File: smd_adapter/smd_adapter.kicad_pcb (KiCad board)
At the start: 2 copper layers, 63.9 x 74.2 mm, 260 parts, among them J1 Conn_01x01_Pin, J10 Conn_01x01_Pin, J11 Conn_01x01_Pin, J12 Conn_01x01_Pin, J13 Conn_01x01_Pin, J14 Conn_01x01_Pin, J15 Conn_01x01_Pin, J16 Conn_01x01_Pin, J17 Conn_01x01_Pin, J18 Conn_01x01_Pin, J19 Conn_01x01_Pin, J2 Conn_01x01_Pin, J20 Conn_01x01_Pin, J21 Conn_01x01_Pin, J22 Conn_01x01_Pin, J23 Conn_01x01_Pin, J24 Conn_01x01_Pin, J25 Conn_01x01_Pin, J26 Conn_01x01_Pin, J27 Conn_01x01_Pin, J28 Conn_01x01_Pin, J29 Conn_01x01_Pin, J3 Conn_01x01_Pin, J30 Conn_01x01_Pin, J31 Conn_01x01_Pin, J32 Conn_01x01_Pin, J33 Conn_01x01_Pin, J34 Conn_01x01_Pin, J35 Conn_01x01_Pin, J36 Conn_01x01_Pin, J37 Conn_01x01_Pin, J4 Conn_01x01_Pin, J5 Conn_01x01_Pin, J6 Conn_01x01_Pin, J7 Conn_01x01_Pin, J8 Conn_01x01_Pin, J9 Conn_01x01_Pin, U1 SOIC8, U2 SOT_32-5, U3 SOT_32-6, U4 MSOP8, U5 TSSOP-10

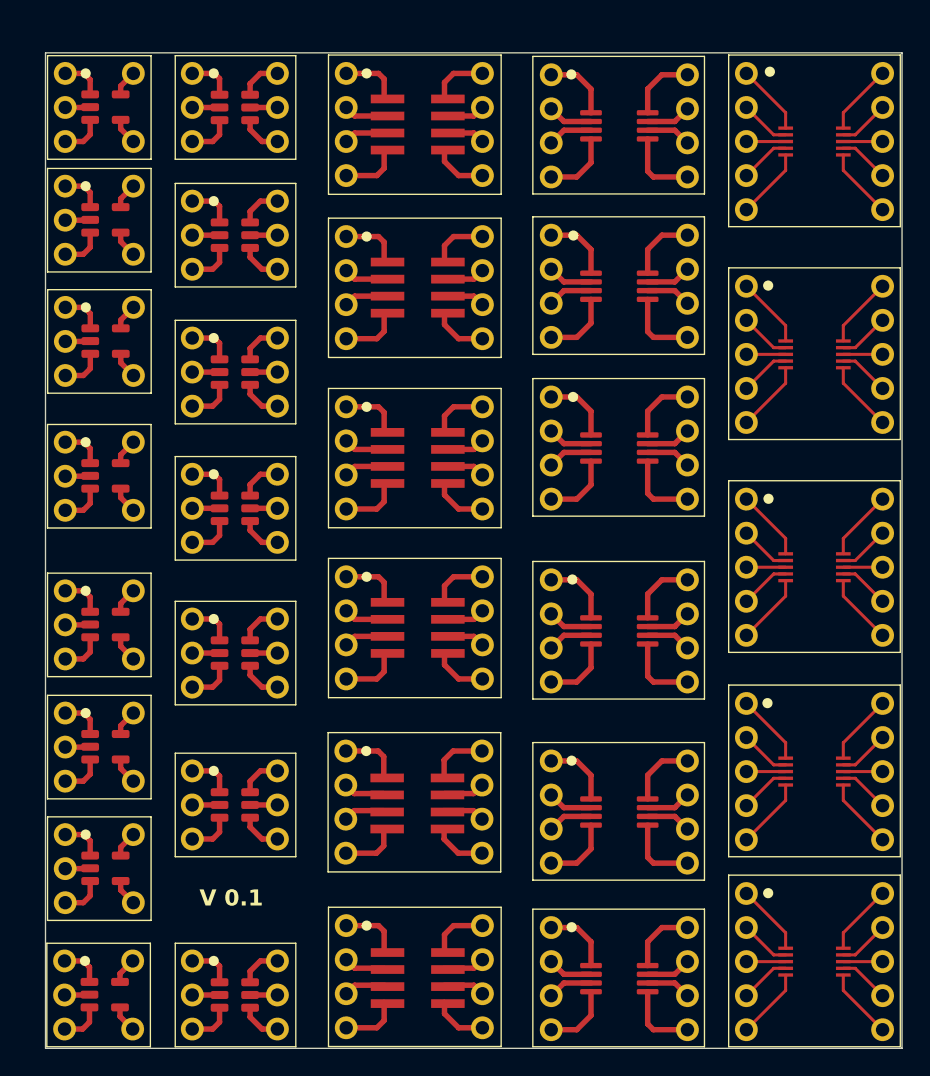
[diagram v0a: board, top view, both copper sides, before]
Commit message: Generated production files.
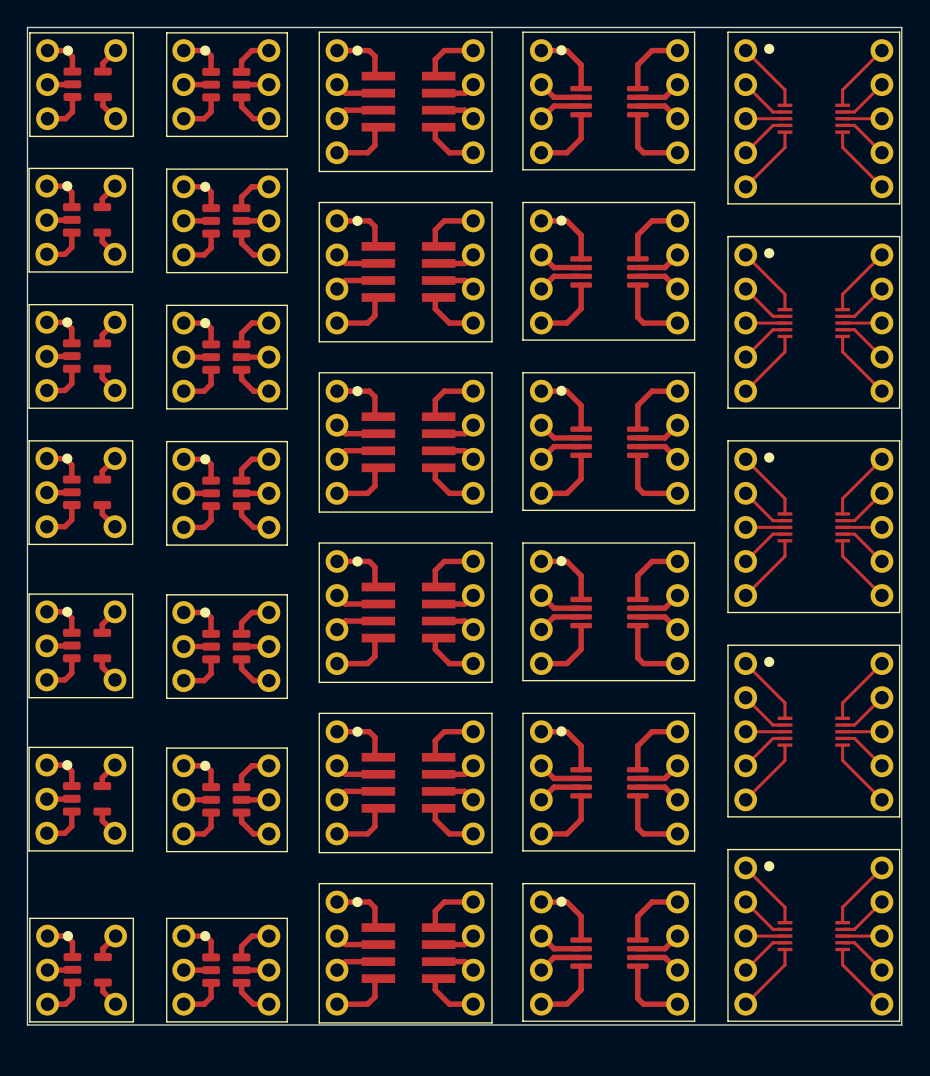
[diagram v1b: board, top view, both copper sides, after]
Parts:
- removed the J1 at (87.7, 107.8)
- removed the J1 at (87.6, 126.3)
- removed the J1 at (87.7, 87.6)
- removed the J1 at (87.7, 68.5)
- removed the J1 at (87.7, 98.7)
- removed the J1 at (87.7, 116.9)
- removed the J1 at (87.7, 77.6)
- removed the J10 at (113.7, 105.6)
- removed the J10 at (113.7, 118.6)
- removed the J10 at (113.7, 79.9)
- removed the J10 at (113.7, 92.6)
- removed the J10 at (113.7, 67.2)
- removed the J11 at (113.7, 82.4)
- removed the J11 at (113.7, 95.1)
- removed the J11 at (113.7, 69.7)
- removed the J11 at (113.7, 121.1)
- removed the J11 at (113.7, 108.1)
- removed the J12 at (113.7, 110.7)
- removed the J12 at (113.7, 85.0)
- removed the J12 at (113.7, 97.7)
- removed the J12 at (113.7, 72.3)
- removed the J12 at (113.7, 123.7)
- removed the J13 at (113.7, 113.2)
- removed the J13 at (113.7, 87.5)
- removed the J13 at (113.7, 74.8)
- removed the J13 at (113.7, 100.2)
- removed the J13 at (113.7, 126.2)
- removed the J14 at (92.1, 121.2)
- removed the J14 at (92.1, 64.6)
- removed the J14 at (92.1, 95.7)
- removed the J14 at (92.1, 107.1)
- removed the J14 at (92.1, 74.8)
- removed the J14 at (92.1, 84.9)
- removed the J15 at (92.1, 98.3)
- removed the J15 at (92.1, 109.6)
- removed the J15 at (92.1, 123.8)
- removed the J15 at (92.1, 77.3)
- removed the J15 at (92.1, 87.5)
- removed the J15 at (92.1, 67.1)
- removed the J16 at (92.1, 112.1)
- removed the J16 at (92.1, 126.3)
- removed the J16 at (92.1, 69.6)
- removed the J16 at (92.1, 90.0)
- removed the J16 at (92.1, 79.9)
- removed the J16 at (92.1, 100.8)
- removed the J17 at (98.4, 74.8)
- removed the J17 at (98.4, 121.2)
- removed the J17 at (98.4, 95.7)
- removed the J17 at (98.4, 84.9)
- removed the J17 at (98.4, 64.6)
- removed the J17 at (98.4, 107.1)
- removed the J18 at (98.4, 109.6)
- removed the J18 at (98.4, 77.3)
- removed the J18 at (98.4, 98.3)
- removed the J18 at (98.4, 123.8)
- removed the J18 at (98.4, 87.5)
- removed the J18 at (98.4, 67.1)
- removed the J19 at (98.4, 100.8)
- removed the J19 at (98.4, 126.3)
- removed the J19 at (98.4, 79.9)
- removed the J19 at (98.4, 69.6)
- removed the J19 at (98.4, 90.0)
- removed the J19 at (98.4, 112.1)
- removed the J2 at (87.7, 72.5)
- removed the J2 at (87.7, 82.5)
- removed the J2 at (87.7, 63.4)
- removed the J2 at (87.7, 93.6)
- removed the J2 at (87.6, 121.2)
- removed the J2 at (87.7, 102.7)
- removed the J2 at (87.7, 111.8)
- removed the J20 at (118.8, 79.2)
- removed the J20 at (118.8, 67.1)
- removed the J20 at (118.8, 118.7)
- removed the J20 at (118.8, 106.3)
- removed the J20 at (118.8, 92.8)
- removed the J21 at (118.8, 81.7)
- removed the J21 at (118.8, 69.6)
- removed the J21 at (118.8, 108.9)
- removed the J21 at (118.8, 95.4)
- removed the J21 at (118.8, 121.3)
- removed the J22 at (118.8, 123.8)
- removed the J22 at (118.8, 111.4)
- removed the J22 at (118.8, 97.9)
- removed the J22 at (118.8, 84.3)
- removed the J22 at (118.8, 72.2)
- removed the J23 at (118.8, 126.4)
- removed the J23 at (118.8, 74.7)
- removed the J23 at (118.8, 86.8)
- removed the J23 at (118.8, 100.4)
- removed the J23 at (118.8, 113.9)
- removed the J24 at (129.0, 118.7)
- removed the J24 at (129.0, 67.1)
- removed the J24 at (129.0, 106.3)
- removed the J24 at (129.0, 79.2)
- removed the J24 at (129.0, 92.8)
- removed the J25 at (129.0, 81.7)
- removed the J25 at (129.0, 95.4)
- removed the J25 at (129.0, 69.6)
- removed the J25 at (129.0, 121.3)
- removed the J25 at (129.0, 108.9)
- removed the J26 at (129.0, 123.8)
- removed the J26 at (129.0, 97.9)
- removed the J26 at (129.0, 72.2)
- removed the J26 at (129.0, 111.4)
- removed the J26 at (129.0, 84.3)
- removed the J27 at (129.0, 86.8)
- removed the J27 at (129.0, 126.4)
- removed the J27 at (129.0, 74.7)
- removed the J27 at (129.0, 113.9)
- removed the J27 at (129.0, 100.4)
- removed the J28 at (133.4, 70.9)
- removed the J28 at (133.4, 86.8)
- removed the J28 at (133.4, 116.2)
- removed the J28 at (133.4, 102.0)
- removed the J29 at (133.4, 104.6)
- removed the J29 at (133.4, 118.7)
- removed the J29 at (133.4, 73.5)
- removed the J29 at (133.4, 89.3)
- removed the J3 at (82.6, 96.2)
- removed the J3 at (82.6, 114.4)
- removed the J3 at (82.6, 75.0)
- removed the J3 at (82.6, 66.0)
- removed the J3 at (82.5, 123.8)
- removed the J3 at (82.6, 105.3)
- removed the J3 at (82.6, 85.1)
- removed the J30 at (133.4, 107.1)
- removed the J30 at (133.4, 91.9)
- removed the J30 at (133.4, 121.3)
- removed the J30 at (133.4, 76.0)
- removed the J31 at (133.4, 109.7)
- removed the J31 at (133.4, 123.8)
- removed the J31 at (133.4, 94.4)
- removed the J31 at (133.4, 78.5)
- removed the J32 at (133.4, 81.1)
- removed the J32 at (133.4, 126.4)
- removed the J32 at (133.4, 112.2)
- removed the J32 at (133.4, 97.0)
- removed the J33 at (143.6, 102.0)
- removed the J33 at (143.6, 116.2)
- removed the J33 at (143.6, 70.9)
- removed the J33 at (143.6, 86.8)
- removed the J34 at (143.6, 118.7)
- removed the J34 at (143.6, 104.6)
- removed the J34 at (143.6, 89.3)
- removed the J34 at (143.6, 73.5)
- removed the J35 at (143.6, 121.3)
- removed the J35 at (143.6, 91.9)
- removed the J35 at (143.6, 107.1)
- removed the J35 at (143.6, 76.0)
- removed the J36 at (143.6, 78.5)
- removed the J36 at (143.6, 109.7)
- removed the J36 at (143.6, 123.8)
- removed the J36 at (143.6, 94.4)
- removed the J37 at (143.6, 112.2)
- removed the J37 at (143.6, 126.4)
- removed the J37 at (143.6, 97.0)
- removed the J37 at (143.6, 81.1)
- removed the J4 at (82.6, 102.7)
- removed the J4 at (82.6, 111.8)
- removed the J4 at (82.6, 63.4)
- removed the J4 at (82.5, 121.2)
- removed the J4 at (82.6, 82.5)
- removed the J4 at (82.6, 72.5)
- removed the J4 at (82.6, 93.6)
- removed the J5 at (82.6, 87.6)
- removed the J5 at (82.6, 116.9)
- removed the J5 at (82.6, 68.5)
- removed the J5 at (82.6, 77.6)
- removed the J5 at (82.6, 98.7)
- removed the J5 at (82.5, 126.3)
- removed the J5 at (82.6, 107.8)
- removed the J6 at (103.5, 105.6)
- removed the J6 at (103.6, 67.2)
- removed the J6 at (103.6, 92.6)
- removed the J6 at (103.6, 118.6)
- removed the J6 at (103.6, 79.9)
- removed the J7 at (103.6, 121.1)
- removed the J7 at (103.5, 108.1)
- removed the J7 at (103.6, 95.1)
- removed the J7 at (103.6, 69.7)
- removed the J7 at (103.6, 82.4)
- removed the J8 at (103.6, 123.7)
- removed the J8 at (103.5, 110.7)
- removed the J8 at (103.6, 85.0)
- removed the J8 at (103.6, 97.7)
- removed the J8 at (103.6, 72.3)
- removed the J9 at (103.5, 113.2)
- removed the J9 at (103.6, 74.8)
- removed the J9 at (103.6, 87.5)
- removed the J9 at (103.6, 100.2)
- removed the J9 at (103.6, 126.2)
- removed the U1 at (108.9, 71.0)
- removed the U1 at (108.9, 109.5)
- removed the U1 at (108.9, 122.5)
- removed the U1 at (108.9, 83.7)
- removed the U1 at (108.9, 96.4)
- removed the U2 at (85.6, 85.1)
- removed the U2 at (85.6, 114.3)
- removed the U2 at (85.5, 123.7)
- removed the U2 at (85.6, 75.0)
- removed the U2 at (85.6, 66.0)
- removed the U2 at (85.6, 105.3)
- removed the U2 at (85.6, 96.1)
- removed the U3 at (95.2, 67.1)
- removed the U3 at (95.2, 98.3)
- removed the U3 at (95.2, 87.5)
- removed the U3 at (95.2, 77.3)
- removed the U3 at (95.2, 123.8)
- removed the U3 at (95.2, 109.6)
- removed U4 (x5): MSOP8, smd_adapter:MSOP-8
- removed the U5 at (138.5, 91.9)
- removed the U5 at (138.5, 76.0)
- removed the U5 at (138.5, 121.3)
- removed the U5 at (138.5, 107.1)
- added J1: Conn_01x01_Pin, smd_adapter:pin_pad, F.Cu at (86.3, 111.7)
- added J1: Conn_01x01_Pin, smd_adapter:pin_pad, F.Cu at (86.3, 100.3)
- added J1: Conn_01x01_Pin, smd_adapter:pin_pad, F.Cu at (86.3, 78.7)
- added J1: Conn_01x01_Pin, smd_adapter:pin_pad, F.Cu at (86.3, 88.8)
- added J1: Conn_01x01_Pin, smd_adapter:pin_pad, F.Cu at (86.4, 124.5)
- added J1: Conn_01x01_Pin, smd_adapter:pin_pad, F.Cu at (86.3, 68.5)
- added J10: Conn_01x01_Pin, smd_adapter:pin_pad, F.Cu at (113.0, 116.8)
- added J10: Conn_01x01_Pin, smd_adapter:pin_pad, F.Cu at (113.0, 66.0)
- added J10: Conn_01x01_Pin, smd_adapter:pin_pad, F.Cu at (113.0, 91.4)
- added J10: Conn_01x01_Pin, smd_adapter:pin_pad, F.Cu at (113.0, 104.1)
- added J10: Conn_01x01_Pin, smd_adapter:pin_pad, F.Cu at (113.0, 78.7)
- added J11: Conn_01x01_Pin, smd_adapter:pin_pad, F.Cu at (113.0, 94.0)
- added J11: Conn_01x01_Pin, smd_adapter:pin_pad, F.Cu at (113.0, 81.3)
- added J11: Conn_01x01_Pin, smd_adapter:pin_pad, F.Cu at (113.0, 106.7)
- added J11: Conn_01x01_Pin, smd_adapter:pin_pad, F.Cu at (113.0, 119.4)
- added J11: Conn_01x01_Pin, smd_adapter:pin_pad, F.Cu at (113.0, 68.6)
- added J12: Conn_01x01_Pin, smd_adapter:pin_pad, F.Cu at (113.0, 121.9)
- added J12: Conn_01x01_Pin, smd_adapter:pin_pad, F.Cu at (113.0, 71.1)
- added J12: Conn_01x01_Pin, smd_adapter:pin_pad, F.Cu at (113.0, 96.5)
- added J12: Conn_01x01_Pin, smd_adapter:pin_pad, F.Cu at (113.0, 83.8)
- added J12: Conn_01x01_Pin, smd_adapter:pin_pad, F.Cu at (113.0, 109.2)
- added J13: Conn_01x01_Pin, smd_adapter:pin_pad, F.Cu at (113.0, 124.5)
- added J13: Conn_01x01_Pin, smd_adapter:pin_pad, F.Cu at (113.0, 73.7)
- added J13: Conn_01x01_Pin, smd_adapter:pin_pad, F.Cu at (113.0, 86.4)
- added J13: Conn_01x01_Pin, smd_adapter:pin_pad, F.Cu at (113.0, 111.8)
- added J13: Conn_01x01_Pin, smd_adapter:pin_pad, F.Cu at (113.0, 99.1)
- added J14: Conn_01x01_Pin, smd_adapter:pin_pad, F.Cu at (91.4, 83.8)
- added J14: Conn_01x01_Pin, smd_adapter:pin_pad, F.Cu at (91.4, 73.7)
- added J14: Conn_01x01_Pin, smd_adapter:pin_pad, F.Cu at (91.4, 63.5)
- added J14: Conn_01x01_Pin, smd_adapter:pin_pad, F.Cu at (91.4, 106.7)
- added J14: Conn_01x01_Pin, smd_adapter:pin_pad, F.Cu at (91.4, 95.2)
- added J14: Conn_01x01_Pin, smd_adapter:pin_pad, F.Cu at (91.4, 119.4)
- added J15: Conn_01x01_Pin, smd_adapter:pin_pad, F.Cu at (91.4, 86.4)
- added J15: Conn_01x01_Pin, smd_adapter:pin_pad, F.Cu at (91.4, 109.2)
- added J15: Conn_01x01_Pin, smd_adapter:pin_pad, F.Cu at (91.4, 97.8)
- added J15: Conn_01x01_Pin, smd_adapter:pin_pad, F.Cu at (91.4, 66.0)
- added J15: Conn_01x01_Pin, smd_adapter:pin_pad, F.Cu at (91.4, 121.9)
- added J15: Conn_01x01_Pin, smd_adapter:pin_pad, F.Cu at (91.4, 76.2)
- added J16: Conn_01x01_Pin, smd_adapter:pin_pad, F.Cu at (91.4, 124.5)
- added J16: Conn_01x01_Pin, smd_adapter:pin_pad, F.Cu at (91.4, 100.3)
- added J16: Conn_01x01_Pin, smd_adapter:pin_pad, F.Cu at (91.4, 111.8)
- added J16: Conn_01x01_Pin, smd_adapter:pin_pad, F.Cu at (91.4, 68.6)
- added J16: Conn_01x01_Pin, smd_adapter:pin_pad, F.Cu at (91.4, 88.9)
- added J16: Conn_01x01_Pin, smd_adapter:pin_pad, F.Cu at (91.4, 78.7)
- added J17: Conn_01x01_Pin, smd_adapter:pin_pad, F.Cu at (97.8, 106.7)
- added J17: Conn_01x01_Pin, smd_adapter:pin_pad, F.Cu at (97.8, 63.5)
- added J17: Conn_01x01_Pin, smd_adapter:pin_pad, F.Cu at (97.8, 119.4)
- added J17: Conn_01x01_Pin, smd_adapter:pin_pad, F.Cu at (97.8, 73.7)
- added J17: Conn_01x01_Pin, smd_adapter:pin_pad, F.Cu at (97.8, 83.8)
- added J17: Conn_01x01_Pin, smd_adapter:pin_pad, F.Cu at (97.8, 95.2)
- added J18: Conn_01x01_Pin, smd_adapter:pin_pad, F.Cu at (97.8, 86.4)
- added J18: Conn_01x01_Pin, smd_adapter:pin_pad, F.Cu at (97.8, 97.8)
- added J18: Conn_01x01_Pin, smd_adapter:pin_pad, F.Cu at (97.8, 76.2)
- added J18: Conn_01x01_Pin, smd_adapter:pin_pad, F.Cu at (97.8, 121.9)
- added J18: Conn_01x01_Pin, smd_adapter:pin_pad, F.Cu at (97.8, 66.0)
- added J18: Conn_01x01_Pin, smd_adapter:pin_pad, F.Cu at (97.8, 109.2)
- added J19: Conn_01x01_Pin, smd_adapter:pin_pad, F.Cu at (97.8, 78.7)
- added J19: Conn_01x01_Pin, smd_adapter:pin_pad, F.Cu at (97.8, 68.6)
- added J19: Conn_01x01_Pin, smd_adapter:pin_pad, F.Cu at (97.8, 124.5)
- added J19: Conn_01x01_Pin, smd_adapter:pin_pad, F.Cu at (97.8, 111.8)
- added J19: Conn_01x01_Pin, smd_adapter:pin_pad, F.Cu at (97.8, 88.9)
- added J19: Conn_01x01_Pin, smd_adapter:pin_pad, F.Cu at (97.8, 100.3)
- added J2: Conn_01x01_Pin, smd_adapter:pin_pad, F.Cu at (86.3, 106.6)
- added J2: Conn_01x01_Pin, smd_adapter:pin_pad, F.Cu at (86.3, 63.4)
- added J2: Conn_01x01_Pin, smd_adapter:pin_pad, F.Cu at (86.3, 73.6)
- added J2: Conn_01x01_Pin, smd_adapter:pin_pad, F.Cu at (86.3, 95.2)
- added J2: Conn_01x01_Pin, smd_adapter:pin_pad, F.Cu at (86.3, 83.8)
- added J2: Conn_01x01_Pin, smd_adapter:pin_pad, F.Cu at (86.4, 119.4)
- added J20: Conn_01x01_Pin, smd_adapter:pin_pad, F.Cu at (118.1, 66.0)
- added J20: Conn_01x01_Pin, smd_adapter:pin_pad, F.Cu at (118.1, 116.8)
- added J20: Conn_01x01_Pin, smd_adapter:pin_pad, F.Cu at (118.1, 78.7)
- added J20: Conn_01x01_Pin, smd_adapter:pin_pad, F.Cu at (118.1, 91.4)
- added J20: Conn_01x01_Pin, smd_adapter:pin_pad, F.Cu at (118.1, 104.1)
- added J21: Conn_01x01_Pin, smd_adapter:pin_pad, F.Cu at (118.1, 94.0)
- added J21: Conn_01x01_Pin, smd_adapter:pin_pad, F.Cu at (118.1, 106.7)
- added J21: Conn_01x01_Pin, smd_adapter:pin_pad, F.Cu at (118.1, 68.6)
- added J21: Conn_01x01_Pin, smd_adapter:pin_pad, F.Cu at (118.1, 81.3)
- added J21: Conn_01x01_Pin, smd_adapter:pin_pad, F.Cu at (118.1, 119.4)
- added J22: Conn_01x01_Pin, smd_adapter:pin_pad, F.Cu at (118.1, 71.1)
- added J22: Conn_01x01_Pin, smd_adapter:pin_pad, F.Cu at (118.1, 96.5)
- added J22: Conn_01x01_Pin, smd_adapter:pin_pad, F.Cu at (118.1, 121.9)
- added J22: Conn_01x01_Pin, smd_adapter:pin_pad, F.Cu at (118.1, 83.8)
- added J22: Conn_01x01_Pin, smd_adapter:pin_pad, F.Cu at (118.1, 109.2)
- added J23: Conn_01x01_Pin, smd_adapter:pin_pad, F.Cu at (118.1, 73.7)
- added J23: Conn_01x01_Pin, smd_adapter:pin_pad, F.Cu at (118.1, 86.4)
- added J23: Conn_01x01_Pin, smd_adapter:pin_pad, F.Cu at (118.1, 124.5)
- added J23: Conn_01x01_Pin, smd_adapter:pin_pad, F.Cu at (118.1, 99.1)
- added J23: Conn_01x01_Pin, smd_adapter:pin_pad, F.Cu at (118.1, 111.8)
- added J24: Conn_01x01_Pin, smd_adapter:pin_pad, F.Cu at (128.3, 78.7)
- added J24: Conn_01x01_Pin, smd_adapter:pin_pad, F.Cu at (128.3, 66.0)
- added J24: Conn_01x01_Pin, smd_adapter:pin_pad, F.Cu at (128.3, 104.1)
- added J24: Conn_01x01_Pin, smd_adapter:pin_pad, F.Cu at (128.3, 91.4)
- added J24: Conn_01x01_Pin, smd_adapter:pin_pad, F.Cu at (128.3, 116.8)
- added J25: Conn_01x01_Pin, smd_adapter:pin_pad, F.Cu at (128.3, 106.7)
- added J25: Conn_01x01_Pin, smd_adapter:pin_pad, F.Cu at (128.3, 81.3)
- added J25: Conn_01x01_Pin, smd_adapter:pin_pad, F.Cu at (128.3, 94.0)
- added J25: Conn_01x01_Pin, smd_adapter:pin_pad, F.Cu at (128.3, 68.6)
- added J25: Conn_01x01_Pin, smd_adapter:pin_pad, F.Cu at (128.3, 119.4)
- added J26: Conn_01x01_Pin, smd_adapter:pin_pad, F.Cu at (128.3, 109.2)
- added J26: Conn_01x01_Pin, smd_adapter:pin_pad, F.Cu at (128.3, 71.1)
- added J26: Conn_01x01_Pin, smd_adapter:pin_pad, F.Cu at (128.3, 96.5)
- added J26: Conn_01x01_Pin, smd_adapter:pin_pad, F.Cu at (128.3, 121.9)
- added J26: Conn_01x01_Pin, smd_adapter:pin_pad, F.Cu at (128.3, 83.8)
- added J27: Conn_01x01_Pin, smd_adapter:pin_pad, F.Cu at (128.3, 124.5)
- added J27: Conn_01x01_Pin, smd_adapter:pin_pad, F.Cu at (128.3, 86.4)
- added J27: Conn_01x01_Pin, smd_adapter:pin_pad, F.Cu at (128.3, 99.1)
- added J27: Conn_01x01_Pin, smd_adapter:pin_pad, F.Cu at (128.3, 73.7)
- added J27: Conn_01x01_Pin, smd_adapter:pin_pad, F.Cu at (128.3, 111.8)
- added J28: Conn_01x01_Pin, smd_adapter:pin_pad, F.Cu at (133.3, 68.6)
- added J28: Conn_01x01_Pin, smd_adapter:pin_pad, F.Cu at (133.3, 99.1)
- added J28: Conn_01x01_Pin, smd_adapter:pin_pad, F.Cu at (133.3, 114.3)
- added J28: Conn_01x01_Pin, smd_adapter:pin_pad, F.Cu at (133.3, 83.8)
- added J29: Conn_01x01_Pin, smd_adapter:pin_pad, F.Cu at (133.3, 101.6)
- added J29: Conn_01x01_Pin, smd_adapter:pin_pad, F.Cu at (133.3, 71.1)
- added J29: Conn_01x01_Pin, smd_adapter:pin_pad, F.Cu at (133.3, 116.8)
- added J29: Conn_01x01_Pin, smd_adapter:pin_pad, F.Cu at (133.3, 86.4)
- added J3: Conn_01x01_Pin, smd_adapter:pin_pad, F.Cu at (81.2, 109.2)
- added J3: Conn_01x01_Pin, smd_adapter:pin_pad, F.Cu at (81.3, 121.9)
- added J3: Conn_01x01_Pin, smd_adapter:pin_pad, F.Cu at (81.2, 86.3)
- added J3: Conn_01x01_Pin, smd_adapter:pin_pad, F.Cu at (81.2, 76.1)
- added J3: Conn_01x01_Pin, smd_adapter:pin_pad, F.Cu at (81.2, 66.0)
- added J3: Conn_01x01_Pin, smd_adapter:pin_pad, F.Cu at (81.2, 97.7)
- added J30: Conn_01x01_Pin, smd_adapter:pin_pad, F.Cu at (133.3, 119.4)
- added J30: Conn_01x01_Pin, smd_adapter:pin_pad, F.Cu at (133.3, 104.1)
- added J30: Conn_01x01_Pin, smd_adapter:pin_pad, F.Cu at (133.3, 88.9)
- added J30: Conn_01x01_Pin, smd_adapter:pin_pad, F.Cu at (133.3, 73.7)
- added J31: Conn_01x01_Pin, smd_adapter:pin_pad, F.Cu at (133.3, 91.4)
- added J31: Conn_01x01_Pin, smd_adapter:pin_pad, F.Cu at (133.3, 106.7)
- added J31: Conn_01x01_Pin, smd_adapter:pin_pad, F.Cu at (133.3, 121.9)
- added J31: Conn_01x01_Pin, smd_adapter:pin_pad, F.Cu at (133.3, 76.2)
- added J32: Conn_01x01_Pin, smd_adapter:pin_pad, F.Cu at (133.3, 94.0)
- added J32: Conn_01x01_Pin, smd_adapter:pin_pad, F.Cu at (133.3, 109.2)
- added J32: Conn_01x01_Pin, smd_adapter:pin_pad, F.Cu at (133.3, 124.5)
- added J32: Conn_01x01_Pin, smd_adapter:pin_pad, F.Cu at (133.3, 78.7)
- added J33: Conn_01x01_Pin, smd_adapter:pin_pad, F.Cu at (143.5, 114.3)
- added J33: Conn_01x01_Pin, smd_adapter:pin_pad, F.Cu at (143.5, 68.6)
- added J33: Conn_01x01_Pin, smd_adapter:pin_pad, F.Cu at (143.5, 99.1)
- added J33: Conn_01x01_Pin, smd_adapter:pin_pad, F.Cu at (143.5, 83.8)
- added J34: Conn_01x01_Pin, smd_adapter:pin_pad, F.Cu at (143.5, 101.6)
- added J34: Conn_01x01_Pin, smd_adapter:pin_pad, F.Cu at (143.5, 116.8)
- added J34: Conn_01x01_Pin, smd_adapter:pin_pad, F.Cu at (143.5, 86.4)
- added J34: Conn_01x01_Pin, smd_adapter:pin_pad, F.Cu at (143.5, 71.1)
- added J35: Conn_01x01_Pin, smd_adapter:pin_pad, F.Cu at (143.5, 119.4)
- added J35: Conn_01x01_Pin, smd_adapter:pin_pad, F.Cu at (143.5, 88.9)
- added J35: Conn_01x01_Pin, smd_adapter:pin_pad, F.Cu at (143.5, 104.1)
- added J35: Conn_01x01_Pin, smd_adapter:pin_pad, F.Cu at (143.5, 73.7)
- added J36: Conn_01x01_Pin, smd_adapter:pin_pad, F.Cu at (143.5, 121.9)
- added J36: Conn_01x01_Pin, smd_adapter:pin_pad, F.Cu at (143.5, 106.7)
- added J36: Conn_01x01_Pin, smd_adapter:pin_pad, F.Cu at (143.5, 76.2)
- added J36: Conn_01x01_Pin, smd_adapter:pin_pad, F.Cu at (143.5, 91.4)
- added J37: Conn_01x01_Pin, smd_adapter:pin_pad, F.Cu at (143.5, 78.7)
- added J37: Conn_01x01_Pin, smd_adapter:pin_pad, F.Cu at (143.5, 94.0)
- added J37: Conn_01x01_Pin, smd_adapter:pin_pad, F.Cu at (143.5, 124.5)
- added J37: Conn_01x01_Pin, smd_adapter:pin_pad, F.Cu at (143.5, 109.2)
- added J4: Conn_01x01_Pin, smd_adapter:pin_pad, F.Cu at (81.2, 73.6)
- added J4: Conn_01x01_Pin, smd_adapter:pin_pad, F.Cu at (81.3, 119.4)
- added J4: Conn_01x01_Pin, smd_adapter:pin_pad, F.Cu at (81.2, 83.8)
- added J4: Conn_01x01_Pin, smd_adapter:pin_pad, F.Cu at (81.2, 106.6)
- added J4: Conn_01x01_Pin, smd_adapter:pin_pad, F.Cu at (81.2, 95.2)
- added J4: Conn_01x01_Pin, smd_adapter:pin_pad, F.Cu at (81.2, 63.4)
- added J5: Conn_01x01_Pin, smd_adapter:pin_pad, F.Cu at (81.2, 100.3)
- added J5: Conn_01x01_Pin, smd_adapter:pin_pad, F.Cu at (81.2, 78.7)
- added J5: Conn_01x01_Pin, smd_adapter:pin_pad, F.Cu at (81.2, 88.8)
- added J5: Conn_01x01_Pin, smd_adapter:pin_pad, F.Cu at (81.2, 68.5)
- added J5: Conn_01x01_Pin, smd_adapter:pin_pad, F.Cu at (81.2, 111.7)
- added J5: Conn_01x01_Pin, smd_adapter:pin_pad, F.Cu at (81.3, 124.5)
- added J6: Conn_01x01_Pin, smd_adapter:pin_pad, F.Cu at (102.9, 104.1)
- added J6: Conn_01x01_Pin, smd_adapter:pin_pad, F.Cu at (102.9, 78.7)
- added J6: Conn_01x01_Pin, smd_adapter:pin_pad, F.Cu at (102.9, 66.0)
- added J6: Conn_01x01_Pin, smd_adapter:pin_pad, F.Cu at (102.9, 91.4)
- added J6: Conn_01x01_Pin, smd_adapter:pin_pad, F.Cu at (102.9, 116.8)
- added J7: Conn_01x01_Pin, smd_adapter:pin_pad, F.Cu at (102.9, 119.4)
- added J7: Conn_01x01_Pin, smd_adapter:pin_pad, F.Cu at (102.9, 68.6)
- added J7: Conn_01x01_Pin, smd_adapter:pin_pad, F.Cu at (102.9, 106.7)
- added J7: Conn_01x01_Pin, smd_adapter:pin_pad, F.Cu at (102.9, 94.0)
- added J7: Conn_01x01_Pin, smd_adapter:pin_pad, F.Cu at (102.9, 81.3)
- added J8: Conn_01x01_Pin, smd_adapter:pin_pad, F.Cu at (102.9, 96.5)
- added J8: Conn_01x01_Pin, smd_adapter:pin_pad, F.Cu at (102.9, 71.1)
- added J8: Conn_01x01_Pin, smd_adapter:pin_pad, F.Cu at (102.9, 109.2)
- added J8: Conn_01x01_Pin, smd_adapter:pin_pad, F.Cu at (102.9, 121.9)
- added J8: Conn_01x01_Pin, smd_adapter:pin_pad, F.Cu at (102.9, 83.8)
- added J9: Conn_01x01_Pin, smd_adapter:pin_pad, F.Cu at (102.9, 124.5)
- added J9: Conn_01x01_Pin, smd_adapter:pin_pad, F.Cu at (102.9, 111.8)
- added J9: Conn_01x01_Pin, smd_adapter:pin_pad, F.Cu at (102.9, 86.4)
- added J9: Conn_01x01_Pin, smd_adapter:pin_pad, F.Cu at (102.9, 73.7)
- added J9: Conn_01x01_Pin, smd_adapter:pin_pad, F.Cu at (102.9, 99.1)
- added U1: SOIC8, smd_adapter:SOIC8, F.Cu at (108.2, 95.2)
- added U1: SOIC8, smd_adapter:SOIC8, F.Cu at (108.2, 108.0)
- added U1: SOIC8, smd_adapter:SOIC8, F.Cu at (108.2, 69.8)
- added U1: SOIC8, smd_adapter:SOIC8, F.Cu at (108.2, 82.5)
- added U1: SOIC8, smd_adapter:SOIC8, F.Cu at (108.2, 120.7)
- added U2: SOT_32-5, smd_adapter:SOT-23-5, F.Cu at (84.3, 121.9)
- added U2: SOT_32-5, smd_adapter:SOT-23-5, F.Cu at (84.2, 86.3)
- added U2: SOT_32-5, smd_adapter:SOT-23-5, F.Cu at (84.2, 109.1)
- added U2: SOT_32-5, smd_adapter:SOT-23-5, F.Cu at (84.2, 66.0)
- added U2: SOT_32-5, smd_adapter:SOT-23-5, F.Cu at (84.2, 97.7)
- added U2: SOT_32-5, smd_adapter:SOT-23-5, F.Cu at (84.2, 76.1)
- added U3: SOT_32-6, smd_adapter:SOT-23-6, F.Cu at (94.6, 66.0)
- added U3: SOT_32-6, smd_adapter:SOT-23-6, F.Cu at (94.6, 121.9)
- added U3: SOT_32-6, smd_adapter:SOT-23-6, F.Cu at (94.6, 86.4)
- added U3: SOT_32-6, smd_adapter:SOT-23-6, F.Cu at (94.6, 109.2)
- added U3: SOT_32-6, smd_adapter:SOT-23-6, F.Cu at (94.6, 76.2)
- added U3: SOT_32-6, smd_adapter:SOT-23-6, F.Cu at (94.6, 97.8)
- added U5: TSSOP-10, smd_adapter:TSSOP-10, F.Cu at (138.4, 88.9)
- added U5: TSSOP-10, smd_adapter:TSSOP-10, F.Cu at (138.4, 73.7)
- added U5: TSSOP-10, smd_adapter:TSSOP-10, F.Cu at (138.4, 104.1)
- added U5: TSSOP-10, smd_adapter:TSSOP-10, F.Cu at (138.4, 119.4)
- added Ue: MSOP8, smd_adapter:MSOP-8, F.Cu at (123.2, 120.7)
- added Ue: MSOP8, smd_adapter:MSOP-8, F.Cu at (123.2, 69.8)
- added Ue: MSOP8, smd_adapter:MSOP-8, F.Cu at (123.2, 108.0)
- added Ue: MSOP8, smd_adapter:MSOP-8, F.Cu at (123.2, 95.2)
- added Ue: MSOP8, smd_adapter:MSOP-8, F.Cu at (123.2, 82.5)
- moved J1 2.15 mm to (86.4, 58.4)
- moved J2 2.15 mm to (86.4, 53.3)
- moved J3 2.15 mm to (81.3, 55.9)
- moved J4 2.15 mm to (81.3, 53.3)
- moved J5 2.15 mm to (81.3, 58.4)
- moved U2 2.15 mm to (84.3, 55.9)
- moved Ue 1.95 mm to (123.2, 57.1)
- moved J20 1.95 mm to (118.1, 53.3)
- moved J21 1.95 mm to (118.1, 55.9)
- moved J22 1.95 mm to (118.1, 58.4)
- moved J23 1.95 mm to (118.1, 61.0)
- moved J24 1.95 mm to (128.3, 53.3)
- moved J25 1.95 mm to (128.3, 55.9)
- moved J26 1.95 mm to (128.3, 58.4)
- moved J27 1.95 mm to (128.3, 61.0)
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- renumbered U4 to Ue
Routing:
- net Net-(J5-Pin_1): track 25.4 -> 22.2 mm
- net Net-(J4-Pin_1): track 25.2 -> 22.1 mm
- net Net-(J1-Pin_1): track 16.1 -> 14.0 mm
- net Net-(J2-Pin_1): track 15.6 -> 13.7 mm
- net Net-(J3-Pin_1): track 15.0 -> 13.1 mm
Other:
- board size 63.9 x 74.2 mm -> 65.2 x 74.4 mm
- board text added: "MSOP-8 0.65mm"
- board text added: "SOIC-8 1.27mm"
- board text added: "SOT23-5 0,95mm"
- board text added: "SOT23-6 0.95mm"
- board text added: "TSSOP-10 0.5mm"
- board text removed: "MSOP-8"
- board text removed: "SOIC-8"
- board text removed: "SOT23-5"
- board text removed: "SOT23-6"
- board text removed: "TSSOP-10"
- board text removed: "V 0.1"
